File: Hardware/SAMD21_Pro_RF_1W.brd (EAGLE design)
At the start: 53.3 x 40.6 mm, 134 parts, among them J10 AVR_SPI_PROG_3X2TESTPOINTS, J12 5.5x2.1mm Barrel, J13 U.FL, J7 PTH, J9 External On/Off, Q1 310mA/60V/1.6Ω, U1 MCP73831, U3 3.3V, U4 ATSAMD21G, U5 4MB Flash, U6 E19-915MS1W, U7 ADJ5, U8 TXB0108DQSR, Y1 32.768kHz

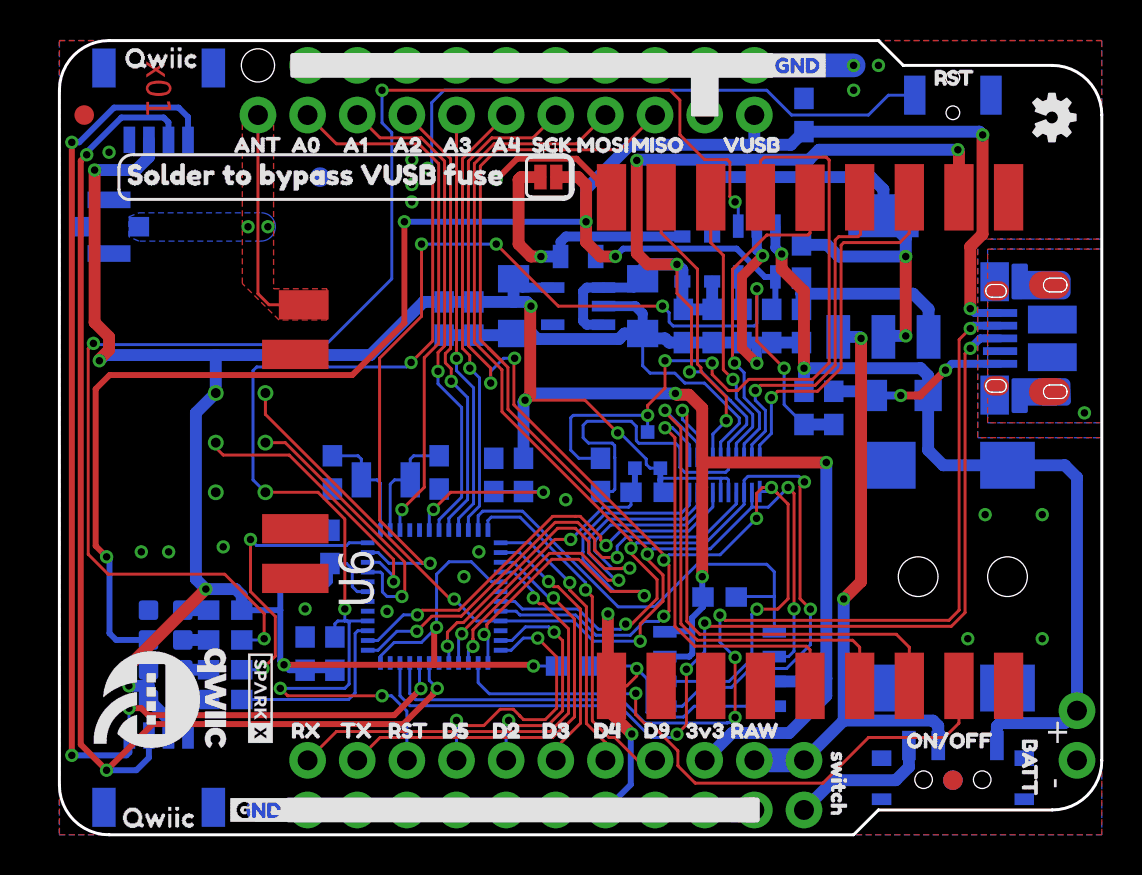
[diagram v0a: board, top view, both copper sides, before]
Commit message: Finalizing things
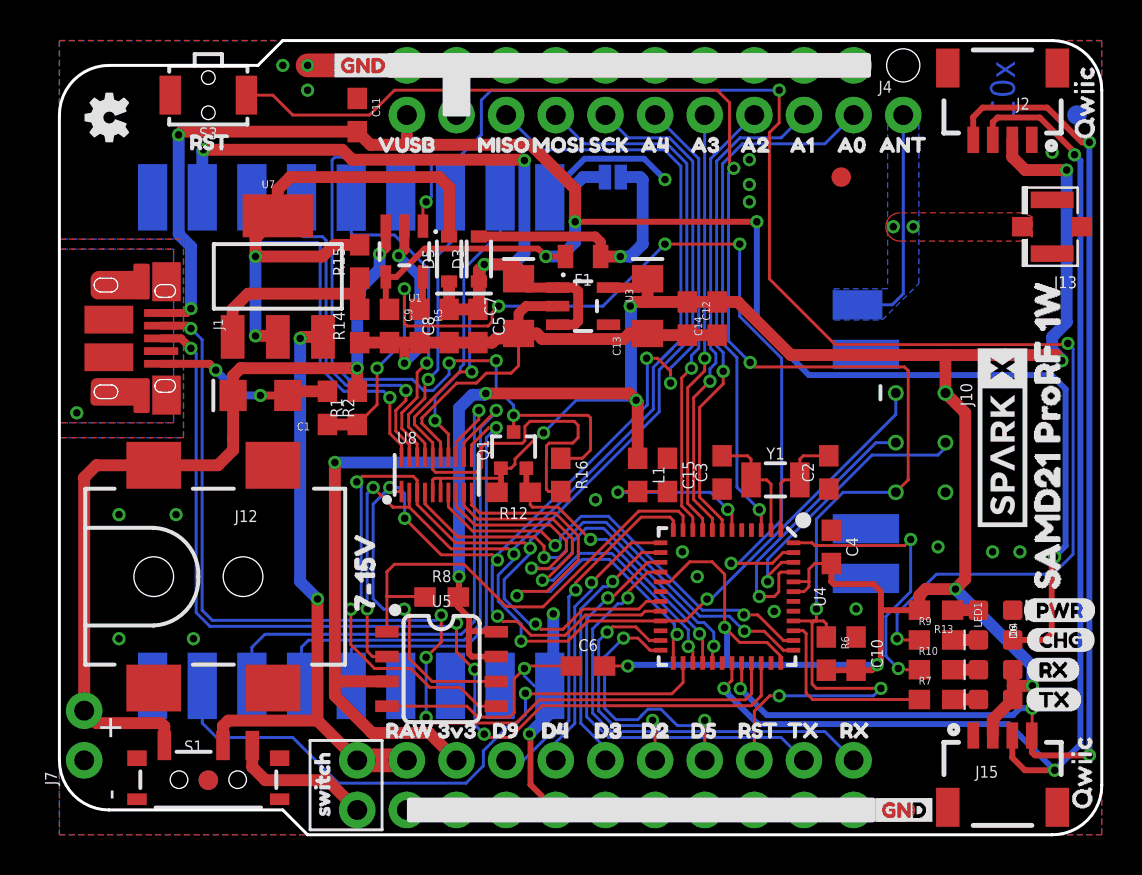
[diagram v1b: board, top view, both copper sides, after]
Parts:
- moved U$26 121.9 mm to (-34.3, -14.0), flipped to the top
- moved FRAME2 81.3 mm to (-14.0, -12.7), flipped to the top
- moved U$29 51.6 mm to (52.5, 34.7), flipped to the top
- moved U$40 51.3 mm to (52.3, 0.38), flipped to the top
- moved FD2 50.8 mm to (52.1, 36.8), flipped to the bottom
- moved J7 50.8 mm to (1.27, 3.81), flipped to the top
- moved U6 50.8 mm to (1.27, 7.62), flipped to the bottom
- moved U$56 48.8 mm to (51.1, 0.89), flipped to the bottom
- moved U$54 48.5 mm to (50.9, 39.8), flipped to the bottom
- moved J13 48.3 mm to (50.8, 31.1), flipped to the top
- moved LOGO1 48.3 mm to (2.54, 36.7), flipped to the bottom
- moved U$35 48.3 mm to (50.8, 33.8), flipped to the bottom
- moved U$61 48.3 mm to (2.54, 36.7), flipped to the top
- moved U$81 47.8 mm to (50.5, 11.4), flipped to the top
- moved U$32 46.0 mm to (3.68, 5.59), flipped to the bottom
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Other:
- outline, holes or cut-outs redrawn

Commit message: x02
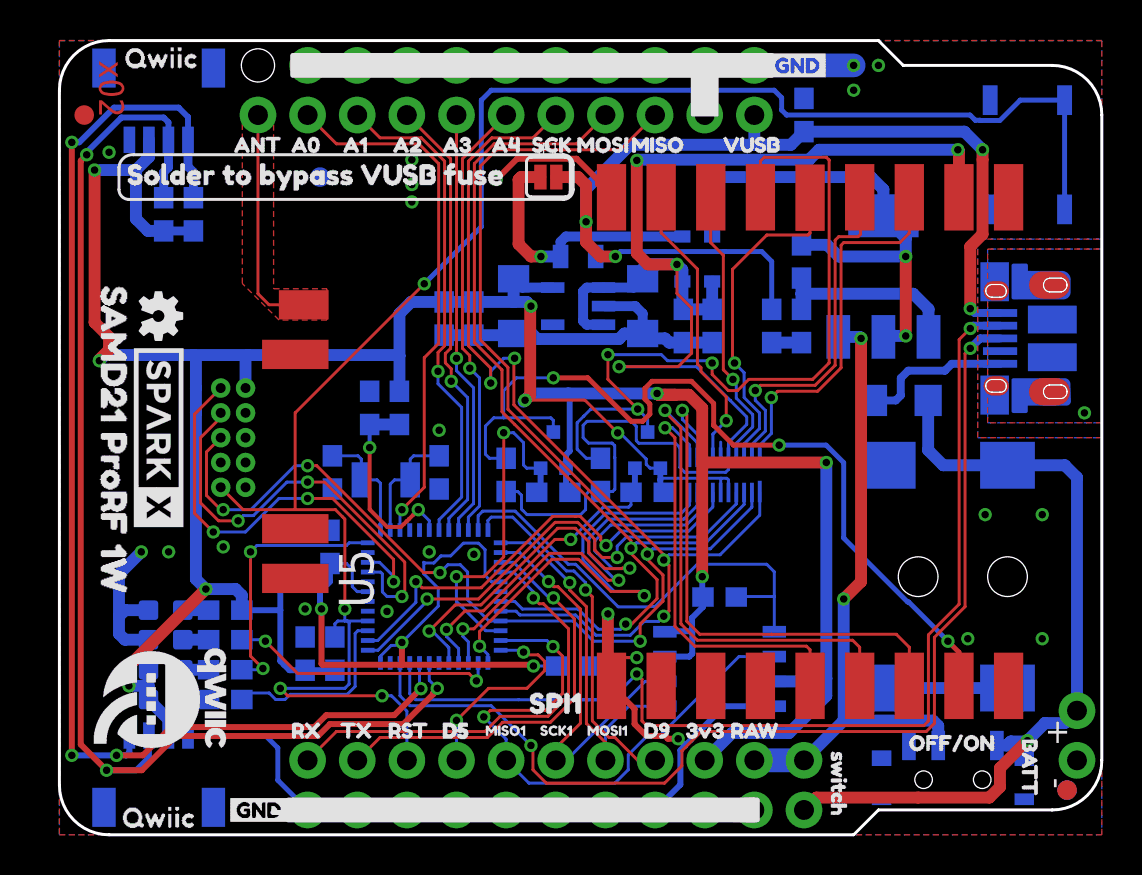
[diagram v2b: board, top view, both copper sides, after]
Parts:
- removed FRAME2: FRAME-LEDGER, SparkFun-Aesthetics:CREATIVE_COMMONS
- removed J15, J2: (no value), SparkFun-Connectors:1X04_1MM_RA
- removed LED1: RED, SparkFun-LED:LED-0603
- removed R15: 240, SparkFun-Resistors:0603
- removed R16: 10k, SparkFun-Resistors:0603
- removed S3: (no value), SparkFun-Switches:TACTILE_SWITCH_SMD_RIGHT_ANGLE
- removed U7: ADJ5, SparkFun-IC-Power:SOT223
- removed U8: TXB0108DQSR, SparkFun-IC-Comms:UFDFN-20
- added D2: Green, SparkFun-LED:LED-0603
- added FRAME1: FRAME-LEDGER, SparkFun-Aesthetics:CREATIVE_COMMONS
- added J14: CORTEX_DEBUG_PTH, SparkFun-Connectors:2X5-PTH-1.27MM
- added Q2: 310mA/60V/1.6Ω, SparkFun-DiscreteSemi:SOT323
- added R11: 10k, SparkFun-Resistors:0603
- added R3, R4: 1k, SparkFun-Resistors:0603
- added S2: Power, SparkFun-Switches:SWITCH_SPST_SMD_A
- added U$58: (no value), SparkX:SPARKX-MEDIUM
- added U$59: (no value), buzzard_labels:D130
- added U$60: (no value), buzzard_labels:SCK18
- added U2: 3.3V, SparkFun-IC-Power:SOT23-5
- C1: value 10uF -> 15pF; device SparkFun-Capacitors:EIA3216 -> SparkFun-Capacitors:0603
- C10: value 0.1uF -> 10uF; device SparkFun-Capacitors:0603 -> SparkFun-Capacitors:EIA3216
- C11, C14: value 0.1uF -> 1.0uF
- C12: value 1.0uF -> 10uF; device SparkFun-Capacitors:0603 -> SparkFun-Capacitors:EIA3216
- C13, C7: value 10uF -> 0.1uF; device SparkFun-Capacitors:EIA3216 -> SparkFun-Capacitors:0603
- C3: value 15pF -> 0.1uF
- C5: value 1.0uF -> 0.1uF
- C8: value 0.1uF -> 4.7uF
- C9: value 4.7uF -> 10uF; device SparkFun-Capacitors:0603 -> SparkFun-Capacitors:EIA3216
- D1: value Green -> Yellow
- D3: value 3A/10V/300mV -> BLUE; device SAMD21_ProRF_1W:SOD-323 -> SparkFun-LED:LED-0603
- D4: value BLUE -> 3A/10V/300mV; device SparkFun-LED:LED-0603 -> SAMD21_ProRF_1W:SOD-323
- D6: value Yellow -> RED
- J10: value AVR_SPI_PROG_3X2TESTPOINTS -> (none); device SparkFun-Connectors:2X3_TEST_POINTS -> SparkFun-Connectors:1X10_NO_SILK
- J11: device SparkFun-Connectors:1X09_NO_SILK -> SparkFun-Connectors:1X04_1MM_RA
- J12: value 5.5x2.1mm Barrel -> (none); device SparkFun-Connectors:POWER_JACK_SMD -> SparkFun-Connectors:1X01_NO_SILK
- J13: value U.FL -> (none); device SparkFun-Connectors:U.FL -> SparkFun-Connectors:1X04_1MM_RA
- J3: value (none) -> PTH; device SparkFun-Connectors:1X10_NO_SILK -> SparkFun-Connectors:1X02_NO_SILK
- J4: device SparkFun-Connectors:1X01_NO_SILK -> SparkFun-Connectors:1X02_NO_SILK
- J5: value (none) -> 5.5x2.1mm Barrel; device SparkFun-Connectors:1X09_NO_SILK -> SparkFun-Connectors:POWER_JACK_SMD
- J7: value PTH -> (none); device SparkFun-Connectors:1X02_NO_SILK -> SparkFun-Connectors:1X09_NO_SILK
- J8: value (none) -> External On/Off
- J9: value External On/Off -> (none); device SparkFun-Connectors:1X02_NO_SILK -> SparkFun-Connectors:1X09_NO_SILK
- R10, R7, R9: value 1k -> 10k
- R13: value 1k -> 2.2k
- R14: value 750 -> 2.2k
- R2, R8: value 10k -> 1k
- R5: value 2.2k -> 240
- R6: value 10k -> 750
- S1: value Power -> MOMENTARY-SWITCH-SPST-SMD-5.2-REDUNDANT; device SparkFun-Switches:SWITCH_SPST_SMD_A -> SparkFun-Switches:TACTILE_SWITCH_SMD_5.2MM
- U$10: device buzzard_labels (25):SCK10 -> buzzard_labels:MISO4
- U$18: device D2:D20 -> buzzard_labels:SCK5
- U$2: device D2:D20 -> buzzard_labels:MISO4
- U$20: device D3:D30 -> buzzard_labels:MOSI3
- U$21: device D3:D30 -> buzzard_labels:SPI11
- U$22: device D4:D40 -> buzzard_labels:MISO17
- U$26: value SPECIAL_INSTRUCTIONS-ORDERING -> (none); device SparkFun-Aesthetics:ORDERING_INSTRUCTIONS -> buzzard_labels:SAMD21_PRORF_1W5
- U$31: device D4:D40 -> buzzard_labels:MOSI16
- U$36: device buzzard_labels (25):RST2 -> buzzard_labels:OFF#ON1
- U$39: device buzzard_labels (28):ON#OFF0 -> buzzard_labels:SCK5
- U$65: device buzzard_labels (9):CHG1 -> buzzard_labels:SPI11
- U$8: device buzzard_labels (25):MISO8 -> buzzard_labels:SPI2
- U$9: device buzzard_labels (25):MOSI9 -> buzzard_labels:MOSI3
- U1: value MCP73831 -> ATSAMD21G; device SparkFun-IC-Power:SOT23-5 -> temp:QFN-48_NO_EXPOSED_PAD
- U3: value 3.3V -> ADJ5; device SparkFun-IC-Power:SOT23-5 -> SparkFun-IC-Power:SOT223
- U4: value ATSAMD21G -> 4MB Flash; device temp:QFN-48_NO_EXPOSED_PAD -> SparkFun-IC-Memory:SO08
- U5: value 4MB Flash -> E19-915MS1W; device SparkFun-IC-Memory:SO08 -> SAMD21_ProRF_1W:E19-915MS1W
- U6: value E19-915MS1W -> TXB0108DQSR; device SAMD21_ProRF_1W:E19-915MS1W -> SparkFun-IC-Comms:UFDFN-20
- moved U$26 56.9 mm to (2.79, 29.2), turned to 270 degrees
- moved S1 52.7 mm to (49.5, 34.8), flipped to the bottom, turned to 270 degrees
- moved J13 52.6 mm to (5.08, 5.08), flipped to the bottom, turned to 0 degrees
- moved U$29 51.6 mm to (0.89, 34.7), flipped to the bottom
- moved U$40 51.3 mm to (1.02, 0.38), flipped to the bottom
- moved U$56 48.8 mm to (2.29, 0.89), flipped to the top
- moved U$54 48.5 mm to (2.41, 39.8), flipped to the top
- moved U$35 48.3 mm to (2.54, 33.8), flipped to the top
- moved U$36 47.8 mm to (42.8, 4.70), flipped to the top
- moved U$81 47.8 mm to (2.79, 11.4), flipped to the bottom
- moved U$28 46.8 mm to (52.7, 33.3), flipped to the bottom, turned to 90 degrees
- moved U$32 46.0 mm to (49.7, 5.59), flipped to the top
- moved J7 45.8 mm to (33.0, 36.8), flipped to the bottom, turned to 0 degrees
- moved U$70 45.5 mm to (3.91, 6.92), flipped to the bottom
- moved U$72 45.5 mm to (3.91, 8.45), flipped to the bottom
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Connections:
- removed net CHARGE_STAT: R9.1, U1.1
- removed net D2: J3.6, U4.23
- removed net D3: J3.5, U4.14
- removed net D4: J3.4, U4.13
- removed net E19_RST: U4.26, U6.P$8
- removed net N$11: R5.1, U1.5
- removed net N$8: D4.C, R9.2
- removed net N$9: J9.2, S1.1
- removed net VBATT_LVL: R1.1, R2.2, U4.47
- new net !E19_RST: Q1.2, R9.1, U1.22
- new net !E19_RST5V: Q1.3, R11.1, U5.P$8
- new net D13: R4.2, U1.26
- new net EEPROM_MISO: J6.6, U1.23, U4.2
- new net EEPROM_MOSI: J6.4, U1.13, U4.5
- new net EEPROM_SCLK: J6.5, U1.14, U4.6
- new net N$3: D3.A, R4.1
- net !E19_CS: now also Q2.2, R10.1, U1.28; no longer Q1.2, R12.1, U4.28
- net !E19_CS5V: now also Q2.3, R12.1, U5.P$15; no longer Q1.3, R16.1, U6.P$15
- net !RST: now also J14.10, J6.8, R1.1, S1.3, S1.4, U1.40; no longer J10.5, J3.8, R6.1, S3.1, U4.40
- net 3.3V: now also C10.+, C11.1, C13.2, C5.2, D2.A, J11.2, J13.2, J14.1, J6.2, Q2.1, R1.2, R10.2, R14.2, R7.2, R9.2, U1.17, U1.36, U1.43, U1.44, U2.5, U4.3, U4.7, U4.8, U6.5, U6.6; no longer C10.2, C12.1, C13.+, C14.2, D6.A, J10.2, J15.2, J2.2, J3.2, R12.2, R6.2, U3.5, U4.17, U4.36, U4.43, U4.44, U5.3, U5.7, U5.8, U8.5, U8.6
- net 5V: now also C12.+, C14.1, C15.2, D4.C, R11.2, R12.2, U2.1, U2.3, U5.P$11, U6.16; no longer C5.1, C7.+, C8.2, D3.C, R16.2, U3.1, U3.3, U6.P$11, U8.16
- net A0: now also J7.9, U1.3; no longer J11.9, U4.3
- net A1: now also J7.8, U1.7; no longer J11.8, U4.7
- net A2: now also J7.7, U1.8; no longer J11.7, U4.8
- net A3: now also J7.6, U1.9; no longer J11.6, U4.9
- net A4: now also J7.5, U1.10; no longer J11.5, U4.10
- net ANT: now also J12.1, U5.P$19; no longer J13.FEED, J4.1, U6.P$19
- net D+: now also U1.34; no longer U4.34
- net D-: now also U1.33; no longer U4.33
- net D10: now also U1.27, U6.9; no longer U4.27, U8.9
- net D11: now also U1.25, U6.10; no longer U4.25, U8.10
- net D5: now also J6.7, U1.24; no longer J3.7, U4.24
- net D8_!FLASH_CS: now also R7.1, U1.11, U4.1; no longer R8.1, U4.11, U5.1
- net D9: now also J6.3, U1.12; no longer J3.3, U4.12
- net DIO05V: now also U5.P$7, U6.13; no longer U6.P$7, U8.13
- net DIO15V: now also U5.P$6, U6.12; no longer U6.P$6, U8.12
- net DIO25V: now also U5.P$5, U6.11; no longer U6.P$5, U8.11
- net E19_INT: now also U1.29, U6.8; no longer U4.29, U8.8
- net E19_RXEN: now also U1.38, U6.7; no longer U4.38, U8.7
- net E19_RXEN5V: now also U5.P$17, U6.14; no longer U6.P$17, U8.14
- net E19_TXEN: now also U1.37, U6.4; no longer U4.37, U8.4
- net E19_TXEN5V: now also U5.P$16, U6.17; no longer U6.P$16, U8.17
- net GND: now also C1.1, C10.-, C11.2, C12.-, C13.1, C14.2, C5.1, C7.1, C8.2, C9.-, D3.C, D6.C, J10.1, J10.10, J10.2, J10.3, J10.4, J10.5, J10.7, J10.8, J10.9, J14.3, J14.5, J3.1, J4.1, J5.GND, J5.P$4, J9.1, J9.2, J9.3, J9.4, J9.5, J9.6, J9.7, J9.8, J9.9, R6.1, S1.1, S1.2, U1.18, U1.35, U1.42, U1.5, U2.2, U4.4, U5.P$1, U5.P$10, U5.P$18, U5.P$20, U5.P$21, U5.P$22, U5.P$9, U6.15; no longer C1.-, C10.1, C11.1, C12.2, C13.-, C14.1, C5.2, C7.-, C8.1, C9.2, J12.GND, J12.P$4, J13.2, J15.1, J2.1, J5.1, J5.2, J5.3, J5.4, J5.5, J5.6, J5.7, J5.8, J5.9, J6.1, J6.10, J6.2, J6.3, J6.4, J6.5, J6.6, J6.7, J6.8, J6.9, J8.1, LED1.C, R14.1, R2.1, R5.2, S3.2, U1.2, U3.2, U4.18, U4.35, U4.42, U4.5, U5.4, U6.P$1, U6.P$10, U6.P$18, U6.P$20, U6.P$21, U6.P$22, U6.P$9, U8.15
- net MISO: now also J14.6, J7.2, U1.21, U6.2; no longer J10.1, J11.2, U4.21, U5.2, U8.2
- net MISO5V: now also U5.P$13, U6.19; no longer U6.P$13, U8.19
- net MOSI: now also J7.3, U1.19, U6.3; no longer J11.3, U4.19, U5.5, U8.3
- net MOSI5V: now also U5.P$14, U6.18; no longer U6.P$14, U8.18
- net N$1: now also D1.C, R2.2; no longer D6.C, R10.2
- net N$12: now also D4.A; no longer D3.A
- net N$13: now also R5.1, R6.2, U3.1; no longer R14.2, R15.1, U7.1
- net N$14: now also R5.2, U3.2, U3.4; no longer R15.2, U7.2, U7.4
- net N$2: now also D2.C, R3.2; no longer D1.C, R7.2
- net N$38: now also D6.A, R8.1; no longer LED1.A, R13.1
- net N$6: now also C1.2, U1.1; no longer C2.2, U4.1
- net N$7: now also C2.2, U1.2; no longer C3.2, U4.2
- net RAW: now also J6.1, J8.1, S2.2, U3.3; no longer J3.1, J9.1, S1.2, U7.3
- net RXI: now also J6.10, U1.16; no longer J3.10, U4.16
- net RX_LED: now also R2.1, U1.48; no longer R10.1, U4.48
- net SCK: now also J7.4, U1.20, U6.1; no longer J11.4, U4.20, U5.6, U8.1
- net SCK5V: now also U5.P$12, U6.20; no longer U6.P$12, U8.20
- net SCL: now also J11.4, J13.4, R14.1, U1.32; no longer J15.4, J2.4, U4.32
- net SDA: now also J11.3, J13.3, R13.1, U1.31; no longer J15.3, J2.3, U4.31
- net SWDCLK: now also J14.4, U1.45; no longer J10.3, U4.45
- net SWDIO: now also J14.2, U1.46; no longer J10.4, U4.46
- net TXO: now also J6.9, U1.15; no longer J3.9, U4.15
- net TX_LED: now also R3.1, U1.39; no longer R7.1, U4.39
- net USB_VCC: now also C3.2, C8.1, J4.2; no longer C11.2, C9.1, D4.A, J8.2, U1.4
- net VBATT: now also C9.+, J3.2, J5.VIN0, J8.2, S2.3; no longer C1.+, J12.VIN0, J7.2, R1.2, S1.3, U1.3
- net VDDANA: now also C7.2, U1.6; no longer C15.2, U4.6
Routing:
- net CHARGE_STAT: track 74.0 -> 0.00 mm, vias 4 -> 0
- net VBATT_LVL: track 52.4 -> 0.00 mm, vias 6 -> 0
- net USB_VCC: track 100.4 -> 53.3 mm, vias 6 -> 4
- net !E19_RST5V: track 0.00 -> 45.1 mm, vias 0 -> 3
- net E19_RST: track 32.0 -> 0.00 mm, vias 1 -> 0
- net EEPROM_MISO: track 0.00 -> 30.0 mm, vias 0 -> 2
- net MOSI: track 71.8 -> 50.4 mm, vias 4 -> 2
- net EEPROM_SCLK: track 0.00 -> 20.8 mm, vias 0 -> 1
- net EEPROM_MOSI: track 0.00 -> 19.3 mm, vias 0 -> 1
- net !E19_RST: track 0.00 -> 18.0 mm, vias 0 -> 2
- net SCK: track 69.6 -> 52.3 mm, vias 7 -> 4
- net 3.3V: track 187.3 -> 204.5 mm
- net D4: track 14.2 -> 0.00 mm, vias 1 -> 0
- net D13: track 0.00 -> 13.8 mm, vias 0 -> 2
- net D3: track 13.5 -> 0.00 mm, vias 1 -> 0
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- removed copper zone on layer 16, net ANT
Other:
- outline, holes or cut-outs redrawn
- board text added: "x02"
- board text removed: "0.8mm Board Thickness"
- board text removed: "x01"

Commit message: x02 ready for order
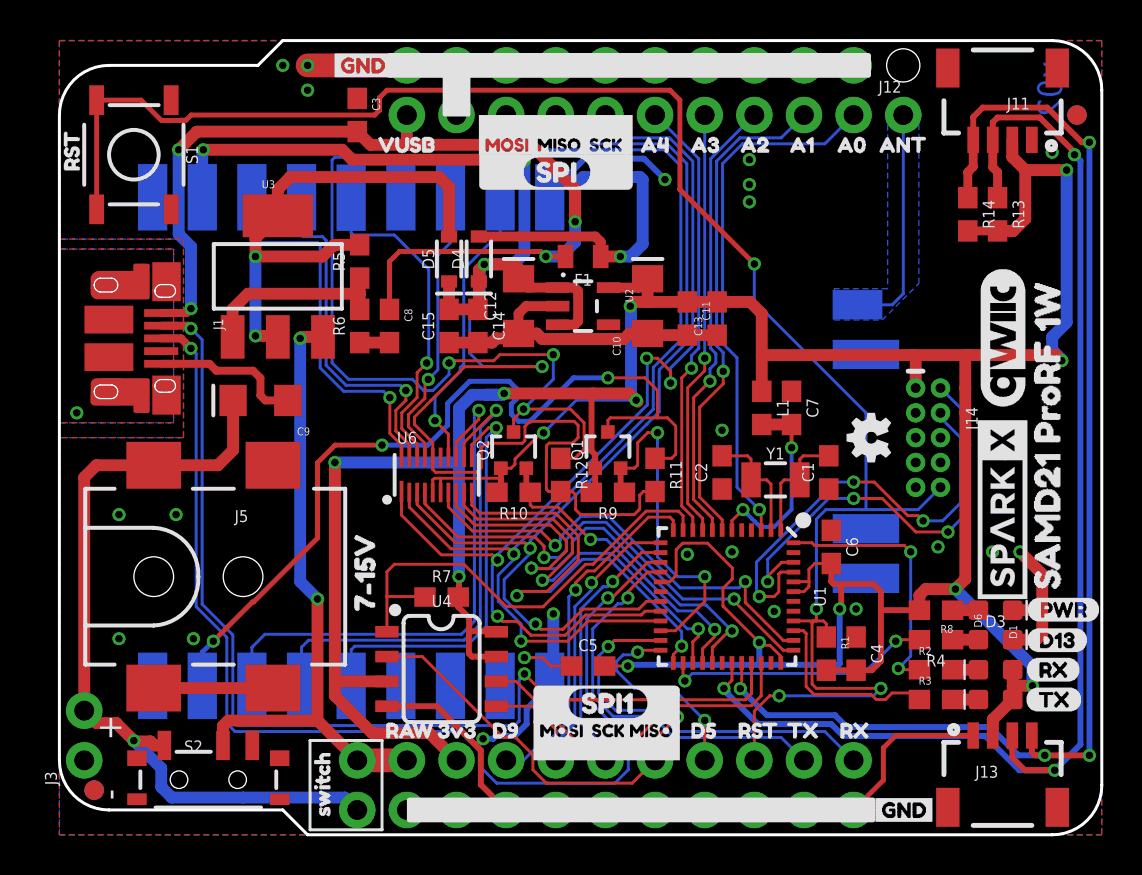
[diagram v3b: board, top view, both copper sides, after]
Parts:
- removed LOGO1: OSHW-LOGOMINI, SparkFun-Aesthetics:OSHW-LOGO-MINI
- removed U$29, U$40, U$54, U$56: (no value), Labels:QWIIC-TEXT-04
- added U$64, U$67: (no value), Labels:QWIIC_COPYRIGHT_SMALL
- U$30: device Labels:QWIIC-LOGO-MEDIUM -> Labels:QWIIC_COPYRIGHT_MEDIUM
- U$34: value SPARKX-LOGO2 -> SPARKX-LOGO4; device SparkX:SPARKX-TINY -> SparkX:SPARKX-MEDIUM
- U$51: device SparkX:SPARKX-MEDIUM -> Labels:QWIIC_COPYRIGHT_MEDIUM
- moved FRAME1 81.3 mm to (-14.0, -12.7), flipped to the top
- moved U$28 52.1 mm to (0.64, 33.3), flipped to the top
- moved FD1 50.8 mm to (52.1, 36.8), flipped to the bottom
- moved J3 50.8 mm to (1.27, 3.81), flipped to the top
- moved U5 50.8 mm to (1.27, 7.62), flipped to the bottom
- moved FD2 49.8 mm to (1.78, 2.29), flipped to the top
- moved FD3 49.8 mm to (1.78, 2.29), flipped to the bottom
- moved U$35 48.3 mm to (50.8, 33.8), flipped to the bottom
- moved U$26 47.8 mm to (50.5, 29.2), flipped to the bottom
- moved U$81 47.8 mm to (50.5, 11.4), flipped to the top
- moved U$32 46.0 mm to (3.68, 5.59), flipped to the bottom
- moved S1 45.7 mm to (3.81, 34.8), flipped to the top
- moved U$63 45.7 mm to (49.5, 11.5), flipped to the top
- moved U$59 45.6 mm to (49.5, 9.96), flipped to the top
- moved U$70 45.5 mm to (49.4, 6.92), flipped to the top
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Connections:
- net GND: now also J14.9
- net MISO: no longer J14.6
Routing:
- net MISO: track 77.3 -> 53.4 mm, vias 5 -> 2
- net GND: track 133.4 -> 132.6 mm
- net 3.3V: track 204.5 -> 203.9 mm
- added copper zone on layer 16, net ANT
- removed copper zone on layer 1, net ANT
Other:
- outline, holes or cut-outs redrawn
